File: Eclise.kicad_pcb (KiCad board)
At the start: 2 copper layers, 101.6 x 101.6 mm, 19 parts, among them J1 Power Supply, J10 Sensor_Power, J11 Sensor_GND, J12 Sensor_Power, J13 Sensor_GND, J14 D12-D13, J2 AMS_In, J3 AMS_Out, J4 Prog_Pins, J5 Prog_Power, J6 A0-A3, J7 A4-A7, J8 D2-D5, J9 D6-D9, U1 ESP-01S

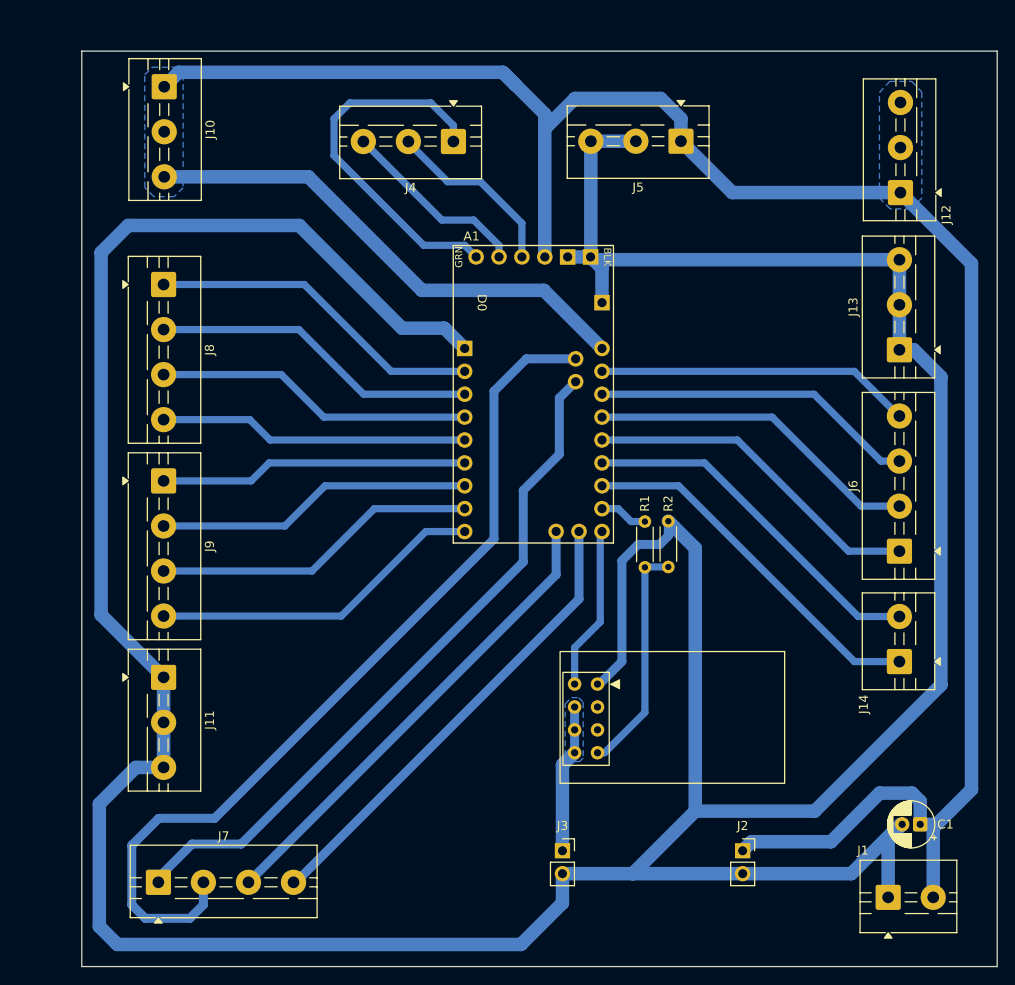
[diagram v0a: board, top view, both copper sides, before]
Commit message: revised pcb
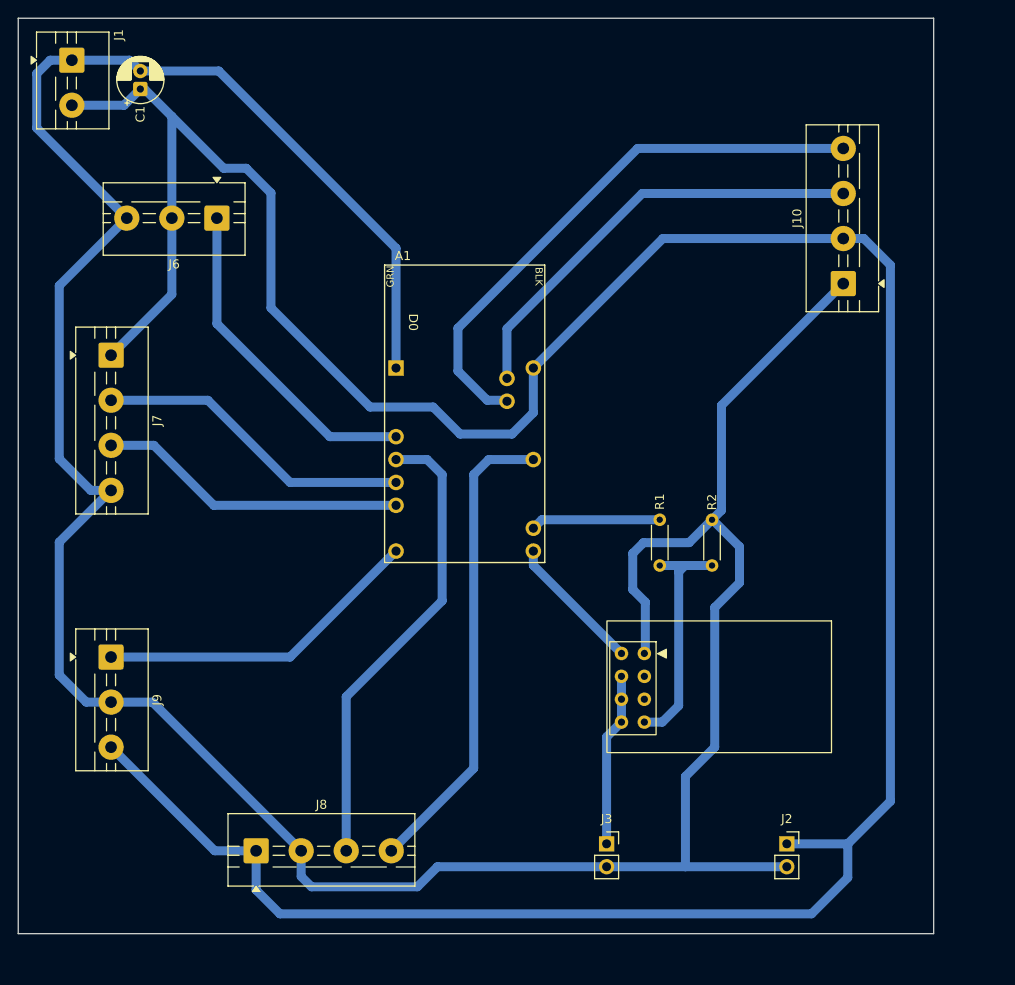
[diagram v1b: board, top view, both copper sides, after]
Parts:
- removed J11, J13: Sensor_GND, TerminalBlock:TerminalBlock_MaiXu_MX126-5.0-03P_1x03_P5.00mm
- removed J12: Sensor_Power, TerminalBlock:TerminalBlock_MaiXu_MX126-5.0-03P_1x03_P5.00mm
- removed J14: D12-D13, TerminalBlock:TerminalBlock_MaiXu_MX126-5.0-02P_1x02_P5.00mm
- removed J4: Prog_Pins, TerminalBlock:TerminalBlock_MaiXu_MX126-5.0-03P_1x03_P5.00mm
- removed J5: Prog_Power, TerminalBlock:TerminalBlock_MaiXu_MX126-5.0-03P_1x03_P5.00mm
- J10: value Sensor_Power -> OLED; footprint TerminalBlock:TerminalBlock_MaiXu_MX126-5.0-03P_1x03_P5.00mm -> TerminalBlock:TerminalBlock_MaiXu_MX126-5.0-04P_1x04_P5.00mm
- J6: value A0-A3 -> DHT; footprint TerminalBlock:TerminalBlock_MaiXu_MX126-5.0-04P_1x04_P5.00mm -> TerminalBlock:TerminalBlock_MaiXu_MX126-5.0-03P_1x03_P5.00mm
- J7: value A4-A7 -> Ultrasonic
- J8: value D2-D5 -> MQ2
- J9: value D6-D9 -> Servo; footprint TerminalBlock:TerminalBlock_MaiXu_MX126-5.0-04P_1x04_P5.00mm -> TerminalBlock:TerminalBlock_MaiXu_MX126-5.0-03P_1x03_P5.00mm
- moved J1 129.8 mm to (87.2, 50.3), turned to -90 degrees
- moved C1 119.0 mm to (94.8, 53.5), turned to 90 degrees
- moved J6 84.3 mm to (103.2, 67.8), turned to 180 degrees
- moved J10 78.5 mm to (172.8, 75.0), turned to 90 degrees
- moved J8 63.7 mm to (107.6, 138.0), turned to 0 degrees
- moved J7 58.7 mm to (91.5, 83.0), turned to -90 degrees
- moved J9 20.4 mm to (91.5, 116.5)
- moved A1 7.92 mm to (130.8, 89.5)
- moved U1 6.21 mm to (150.7, 116.1)
- moved J2 4.96 mm to (166.5, 137.2)
- moved J3 4.96 mm to (146.5, 137.2)
- moved R2 4.85 mm to (158.2, 101.3)
- moved R1 1.66 mm to (152.4, 101.3)
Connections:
- A1 pad A0: Net-(J6-Pin_1) -> MQ2_A0
- A1 pad A4: Net-(A1-A4/SDA) -> OLED_SDA
- A1 pad A5: Net-(A1-A5/SCL) -> OLED_SCL
- A1 pad D4: Net-(J8-Pin_3) -> DHT_Data
- A1 pad D5: Net-(J8-Pin_4) -> MQ2_D5
- A1 pad D6: Net-(J9-Pin_1) -> Trig
- A1 pad D7: Net-(J9-Pin_2) -> Echo
- A1 pad D9: Net-(J9-Pin_4) -> Servo_PWM
- J10 pad 1: 5V -> GND
- J10 pad 3: 5V -> OLED_SCL
- J6 pad 1: Net-(J6-Pin_1) -> DHT_Data
- J6 pad 2: Net-(J6-Pin_2) -> 5V
- J6 pad 3: Net-(J6-Pin_3) -> GND
- J7 pad 1: Net-(A1-A4/SDA) -> 5V
- J7 pad 2: Net-(A1-A5/SCL) -> Trig
- J7 pad 3: Net-(J7-Pin_3) -> Echo
- J7 pad 4: Net-(J7-Pin_4) -> GND
- J8 pad 1: Net-(A1-D2_INT0) -> 5V
- J8 pad 2: Net-(A1-D3_INT1) -> GND
- J8 pad 3: Net-(J8-Pin_3) -> MQ2_D5
- J8 pad 4: Net-(J8-Pin_4) -> MQ2_A0
- J9 pad 1: Net-(J9-Pin_1) -> Servo_PWM
- J9 pad 2: Net-(J9-Pin_2) -> GND
- J9 pad 3: Net-(J9-Pin_3) -> 5V
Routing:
- net GND: track 445.6 -> 332.2 mm
- net Net-(A1-A5/SCL): track 99.5 -> 0.00 mm
- net Net-(A1-A4/SDA): track 77.9 -> 0.00 mm
- net OLED_SDA: track 0.00 -> 62.6 mm
- net Net-(J7-Pin_3): track 53.1 -> 0.00 mm
- net MQ2_A0: track 0.00 -> 52.9 mm
- net Net-(J7-Pin_4): track 52.2 -> 0.00 mm
- net MQ2_D5: track 0.00 -> 52.0 mm
- net 5V: track 275.9 -> 327.7 mm
- net OLED_SCL: track 0.00 -> 49.1 mm
- net /DTR: track 41.3 -> 0.00 mm
- net Net-(A1-D12_MISO): track 41.1 -> 0.00 mm
- net Net-(A1-D13_SCK): track 40.1 -> 0.00 mm
- net Net-(J6-Pin_1): track 38.1 -> 0.00 mm
- net Net-(A1-D2_INT0): track 37.4 -> 0.00 mm
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- removed copper zone on B.Cu, net +3.3V
- removed copper zone on B.Cu, net 5V
